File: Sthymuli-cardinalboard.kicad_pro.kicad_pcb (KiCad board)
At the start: 4 copper layers, 176.5 x 154.2 mm, 41 parts, among them Q10 NX7002AK, Q11 NX7002AK, Q12 NX7002AK, Q13 NX7002AK, SW10 SW_Push, SW7 SW_Push, SW8 SW_Push, SW9 SW_Push, U13 LSM6DS3, U15 ITR9909, U16 ITR9909, U17 ITR9909, U18 ITR9909, U19 ITR9909, U20 ITR9909, U21 ITR9909, U22 ITR9909

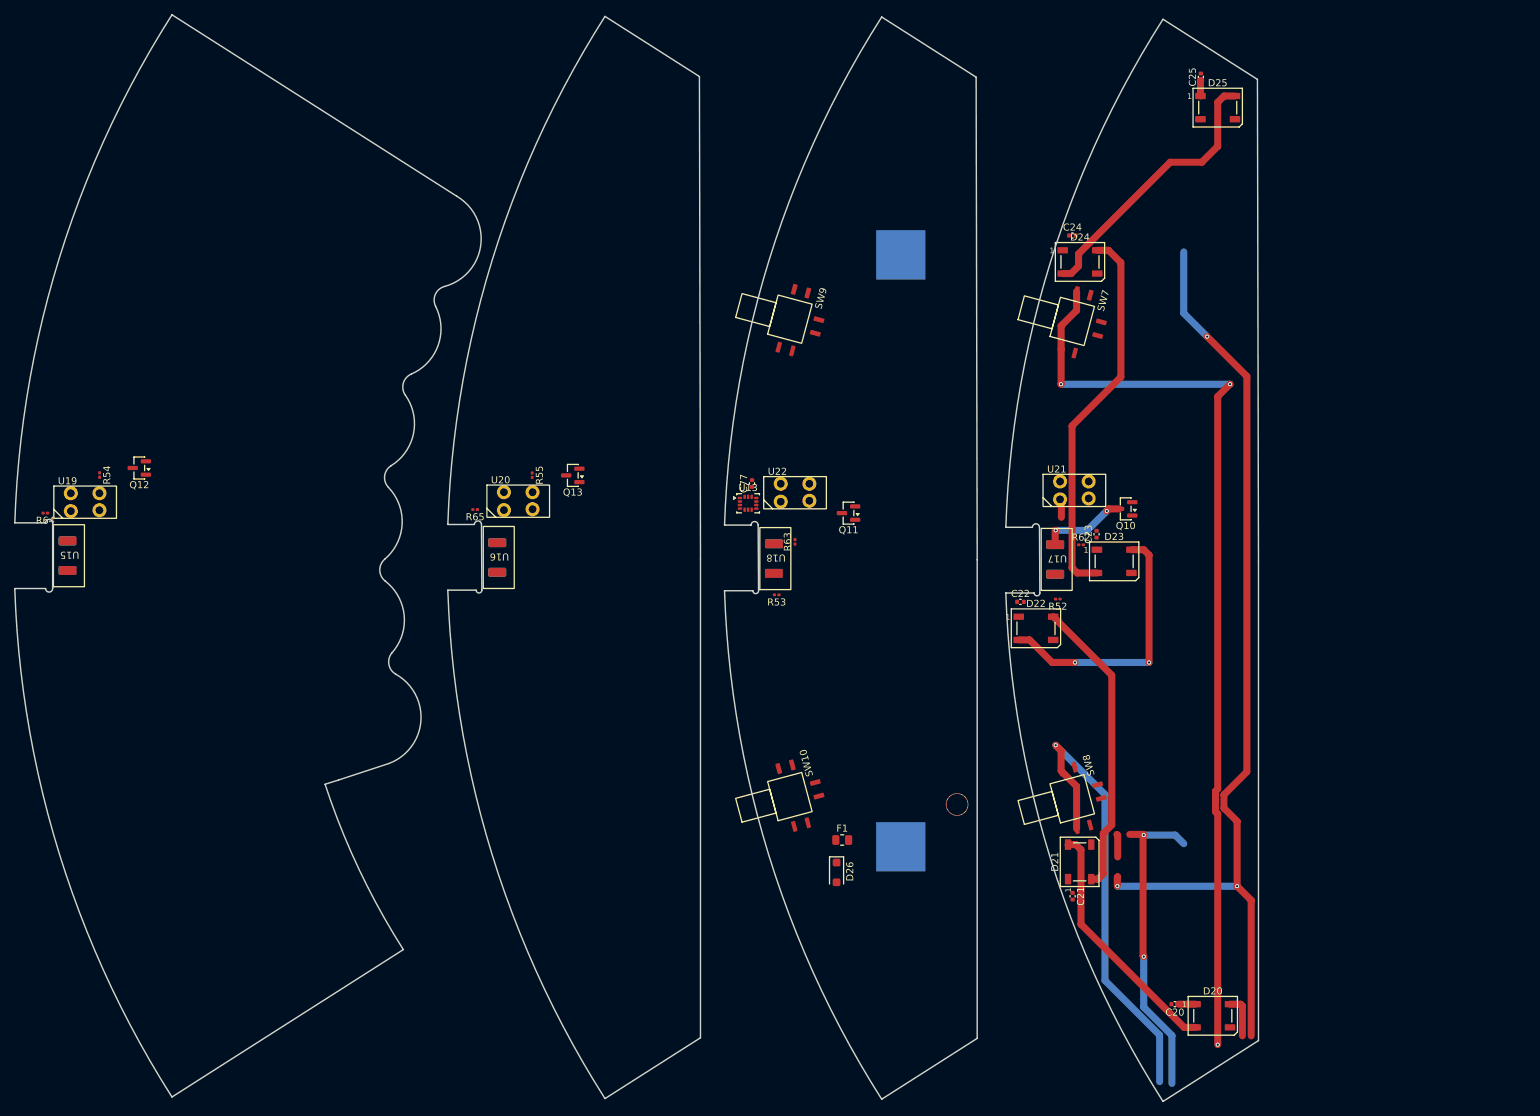
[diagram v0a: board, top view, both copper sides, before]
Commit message: routing small board
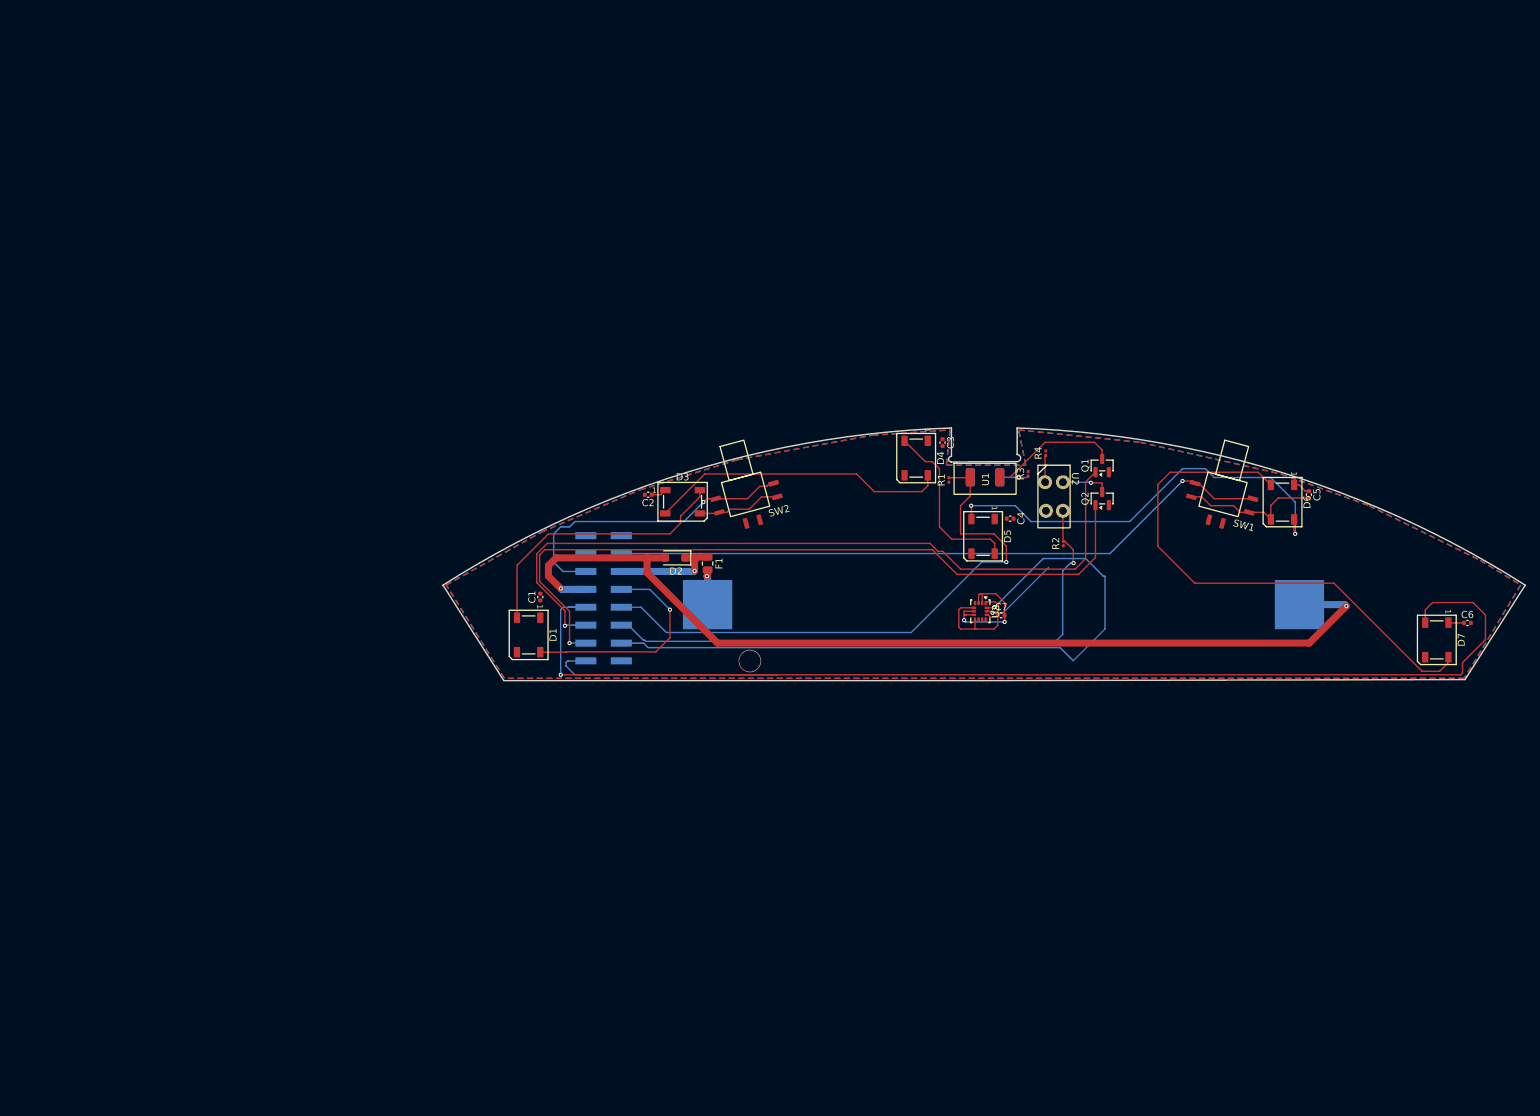
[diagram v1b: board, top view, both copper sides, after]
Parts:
- removed Q12, Q13: NX7002AK, Package_TO_SOT_SMD:SOT-23
- removed R54, R55: 3K3, Capacitor_SMD:C_0201_0603Metric
- removed R64, R65: 27R, Capacitor_SMD:C_0201_0603Metric
- removed SW10, SW9: SW_Push, sthymuli:XKB5858
- removed U15, U16: ITR9909, sthymuli:ITR_9909_Horizontal
- removed U19, U20, U21, U22: ITR9909, sthymuli:ITR_9909_Vertical
- added J1: Conn_02x08_Counter_Clockwise, Connector_PinSocket_2.54mm:PinSocket_2x08_P2.54mm_Vertical_SMD, B.Cu at (96.3, 95.4)
- U2: renamed from U18; footprint sthymuli:ITR_9909_Horizontal -> sthymuli:ITR_9909_Vertical
- moved D1 111.1 mm to (85.7, 100.6), turned to -90 degrees
- moved C1 107.0 mm to (87.3, 95.2), turned to 90 degrees
- moved C6 86.2 mm to (218.9, 98.9), turned to 0 degrees
- moved C2 82.9 mm to (102.7, 80.7), turned to 180 degrees
- moved D7 81.7 mm to (214.6, 101.3), turned to -90 degrees
- moved D3 76.1 mm to (107.5, 81.7), turned to 0 degrees
- moved SW2 63.2 mm to (116.6, 81.1), turned to 15 degrees
- moved D2 50.2 mm to (106.5, 89.7), turned to 180 degrees
- moved C5 49.8 mm to (196.4, 80.7), turned to -90 degrees
- moved D6 44.6 mm to (192.7, 81.7), turned to -90 degrees
- moved F1 43.6 mm to (111.1, 90.5), turned to -90 degrees
- moved R2 41.3 mm to (161.6, 87.6), turned to 90 degrees
- moved U2 40.7 mm to (160.3, 80.9), turned to -90 degrees
- moved C7 40.0 mm to (152.8, 97.8), turned to 0 degrees
- moved R4 37.8 mm to (159.1, 74.8)
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- renumbered C20 to C1, C21 to C2, C22 to C3, C23 to C4, C24 to C5, C25 to C6, C77 to C7, D20 to D1, D26 to D2, D21 to D3, D22 to D4, D23 to D5, D24 to D6, D25 to D7, Q10 to Q1, Q11 to Q2, R52 to R1, R53 to R2, R62 to R3, R63 to R4, SW7 to SW1, SW8 to SW2, U17 to U1, U13 to U3
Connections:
- net IR_REC_2 renamed IR_REC_HORI
- net IR_REC_3 renamed IR_REC_VERT
- Q1 pad 1: IR_TRA_2 -> IR_TRA_HORI
- Q2 pad 1: IR_TRA_3 -> IR_TRA_VERT
- U3 pad 4: unconnected-(U13-INT1-Pad4) -> ACC_INT
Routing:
- net (no net): track 184.8 -> 0.00 mm, vias 5 -> 0
- net DOUT: track 0.00 -> 164.6 mm, vias 0 -> 1
- net BAT-: track 0.00 -> 139.0 mm, vias 0 -> 2
- net IR_TRA_HORI: track 0.00 -> 108.3 mm, vias 0 -> 1
- net IR_TRA_VERT: track 0.00 -> 105.7 mm, vias 0 -> 1
- net SDA: track 0.00 -> 99.8 mm, vias 0 -> 1
- net IR_REC_VERT: track 0.00 -> 83.2 mm, vias 0 -> 1
- net IR_REC_HORI: track 0.00 -> 81.4 mm, vias 0 -> 1
- net GND: track 0.00 -> 51.8 mm, vias 0 -> 2
- net SCL: track 0.00 -> 45.5 mm, vias 0 -> 1
- net btn_DOWN: track 132.8 -> 94.9 mm, vias 3 -> 1
- net Net-(D6-DOUT): track 39.6 -> 76.1 mm
- net DIN: track 6.10 -> 31.3 mm, vias 0 -> 1
- net btn_UP: track 66.9 -> 43.3 mm
- net +3V3: track 0.00 -> 18.8 mm
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- added copper zone on F.Cu, net +5V
- added copper zone on B.Cu, net GND
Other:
- board size 176.5 x 154.2 mm -> 153.6 x 35.9 mm
- copper layers 4 -> 2
